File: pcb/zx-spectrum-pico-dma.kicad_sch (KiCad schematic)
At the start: 15 parts, among them J101 Conn_Pi_SWD, J102 Conn_01x10, J103 Conn_01x08, J104 Conn_01x16, J105 Conn_01x07, J106 Conn_01x02, J107 Conn_01x04, Q101 PMBT2222A, SW101 BTN_RESET, SW102 BTN_BOOTSEL, SW103 BTN_USR1, SW104 BTN_USR2, U101 RP2350_Stamp_XL

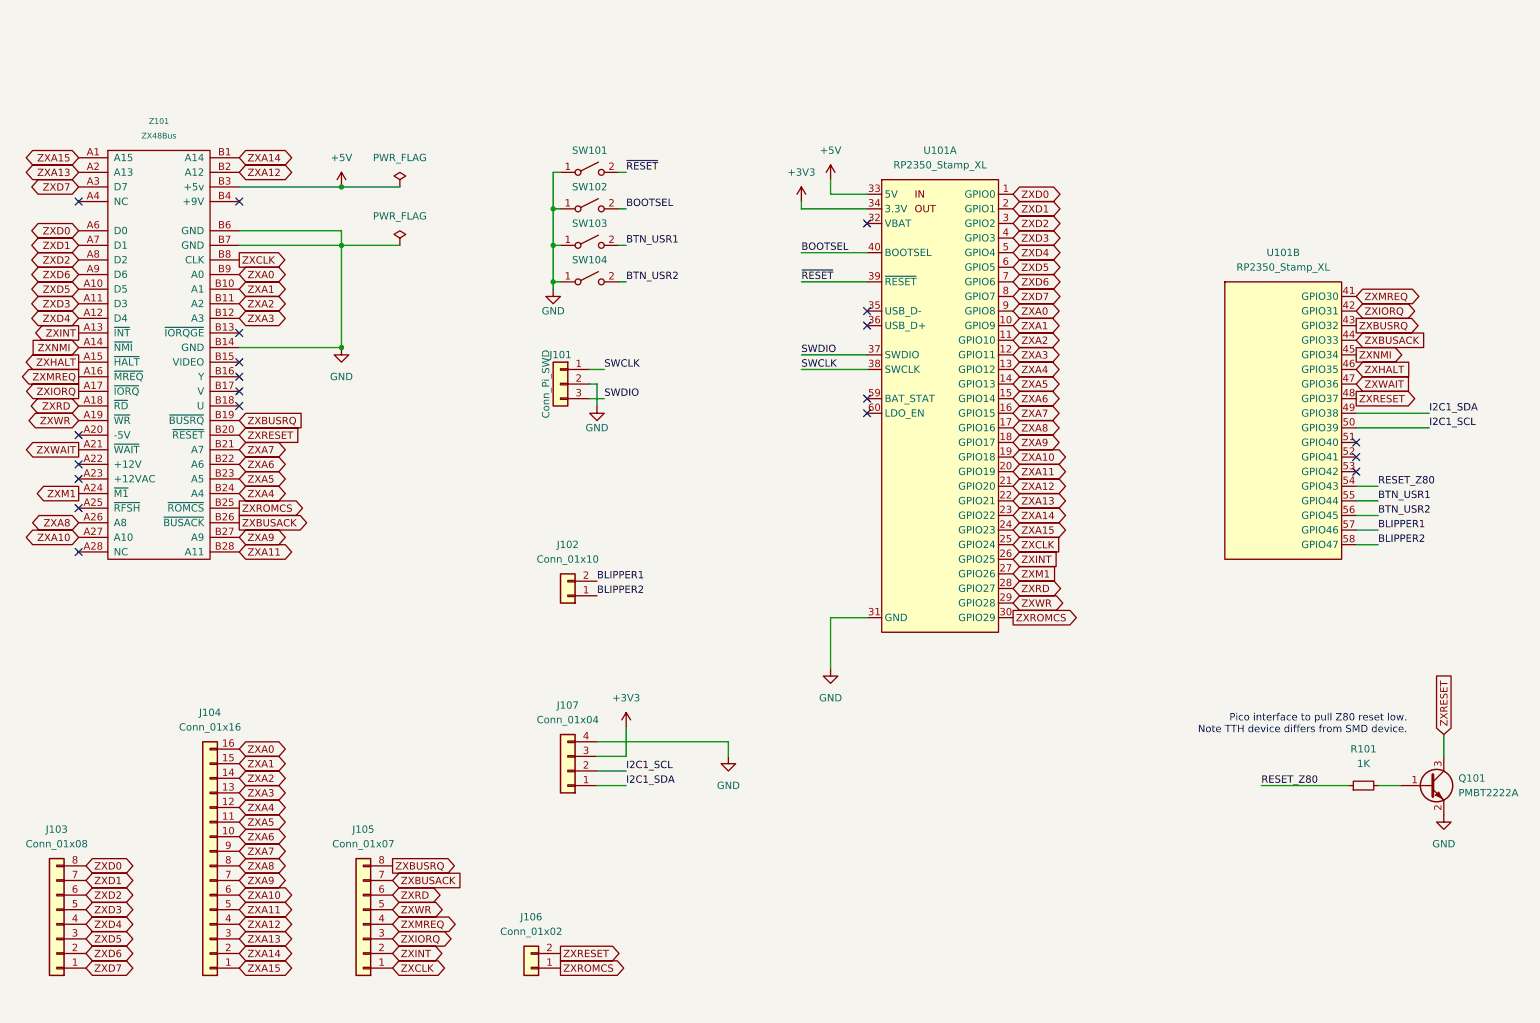
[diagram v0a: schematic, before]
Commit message: more layout work
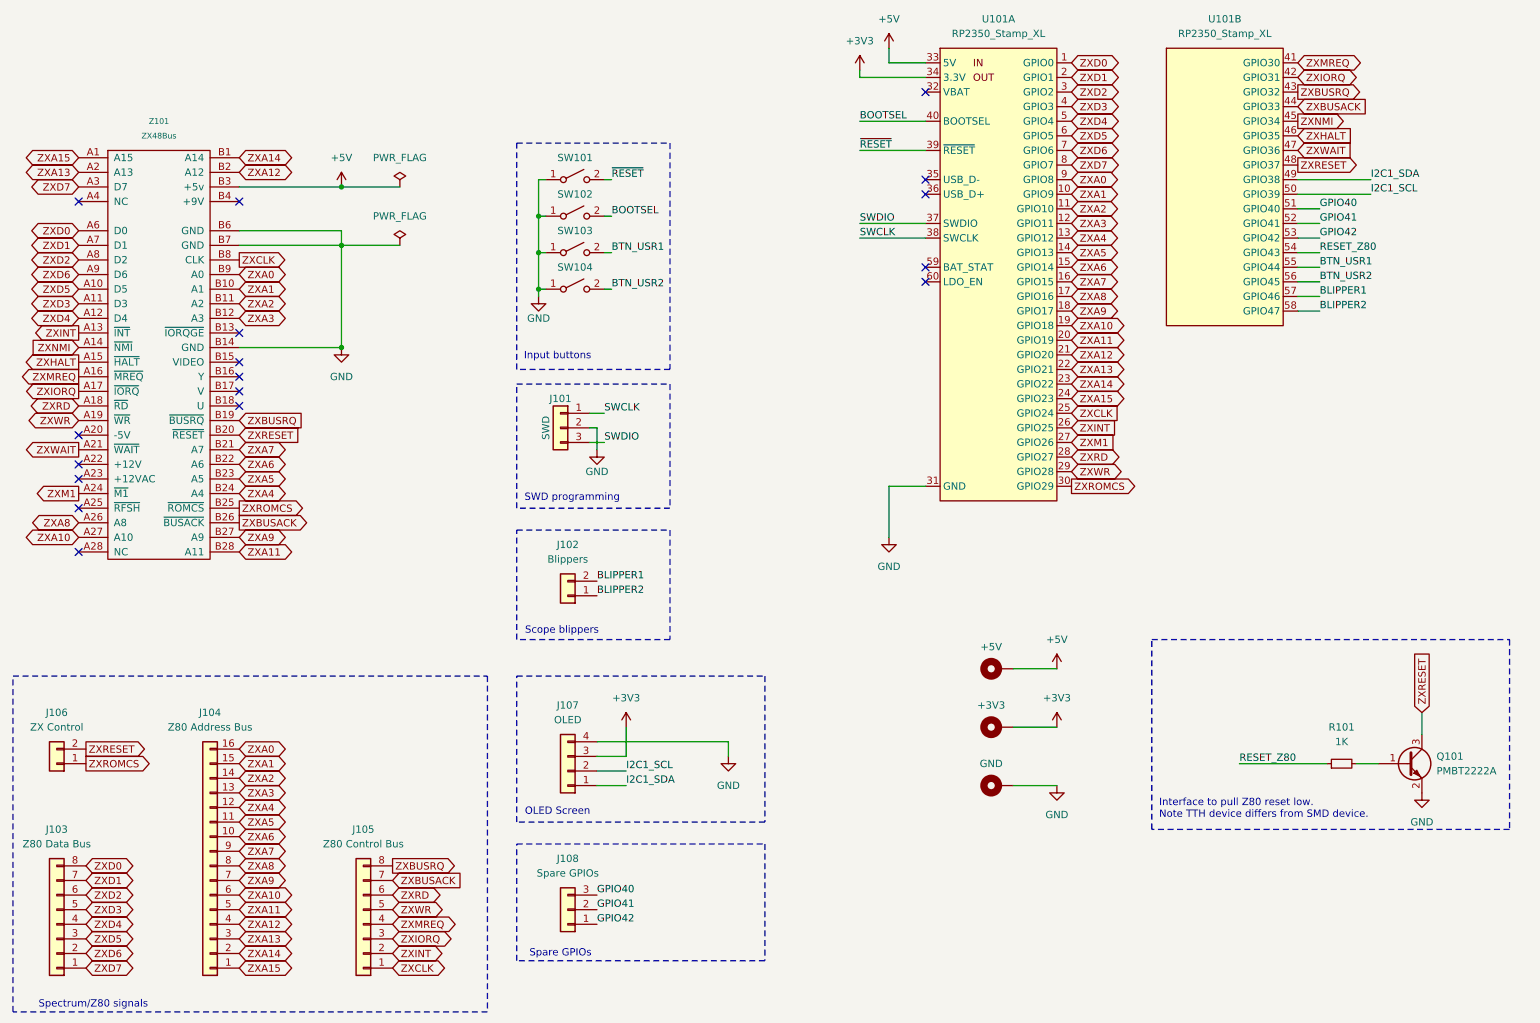
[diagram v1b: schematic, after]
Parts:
- added H101: +5V, MountingHole:MountingHole_2.2mm_M2_Pad, symbol Mechanical:MountingHole_Pad
- added H102: +3V3, MountingHole:MountingHole_2.2mm_M2_Pad, symbol Mechanical:MountingHole_Pad
- added H103: GND, MountingHole:MountingHole_2.2mm_M2_Pad, symbol Mechanical:MountingHole_Pad
- added J108: Spare GPIOs, Connector_PinHeader_2.54mm:PinHeader_1x03_P2.54mm_Vertical, symbol Connector_Generic:Conn_01x03
- J101: value Conn_Pi_SWD -> SWD
- J102: value Conn_01x10 -> Blippers; footprint (none) -> Connector_PinHeader_2.54mm:PinHeader_1x02_P2.54mm_Vertical
- J103: value Conn_01x08 -> Z80 Data Bus; footprint (none) -> Connector_PinHeader_2.54mm:PinHeader_1x08_P2.54mm_Vertical
- J104: value Conn_01x16 -> Z80 Address Bus; footprint (none) -> Connector_PinHeader_2.54mm:PinHeader_1x16_P2.54mm_Vertical
- J105: value Conn_01x07 -> Z80 Control Bus; footprint (none) -> Connector_PinHeader_2.54mm:PinHeader_1x08_P2.54mm_Vertical
- J106: value Conn_01x02 -> ZX Control; footprint (none) -> Connector_PinHeader_2.54mm:PinHeader_1x02_P2.54mm_Vertical
- J107: value Conn_01x04 -> OLED; footprint (none) -> Connector_PinHeader_2.54mm:PinHeader_1x04_P2.54mm_Vertical
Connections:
- net +3V3: now also H102.1
- net +5V: now also H101.1
- net GND: now also H103.1
- net GPIO40: now reaches U101.51 (GPIO40)
- net GPIO40: now also J108.3 (Pin_3)
- net GPIO41: now reaches U101.52 (GPIO41)
- net GPIO41: now also J108.2 (Pin_2)
- net GPIO42: now reaches U101.53 (GPIO42)
- net GPIO42: now also J108.1 (Pin_1)
- no-connect marks 20 -> 17
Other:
- note added: "Input buttons"
- note added: "Interface to pull Z80 reset low. Note TTH device differs from SMD device."
- note added: "OLED Screen"
- note added: "SWD programming"
- note added: "Scope blippers"
- note added: "Spare GPIOs"
- note added: "Spectrum/Z80 signals"
- note removed: "Pico interface to pull Z80 reset low. Note TTH device differs from SMD device."
- title: (none) -> RP2350B Spectrum DMA Interface
- moved on the sheet: J101, J106, Q101, R101, SW101, SW102, SW103, SW104, U101A, U101B
